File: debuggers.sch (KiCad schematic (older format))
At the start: 7 parts, among them P1 TI_JTAG, P2 SWD, P3 TI_jtag, P4 SWD+SWO+UART

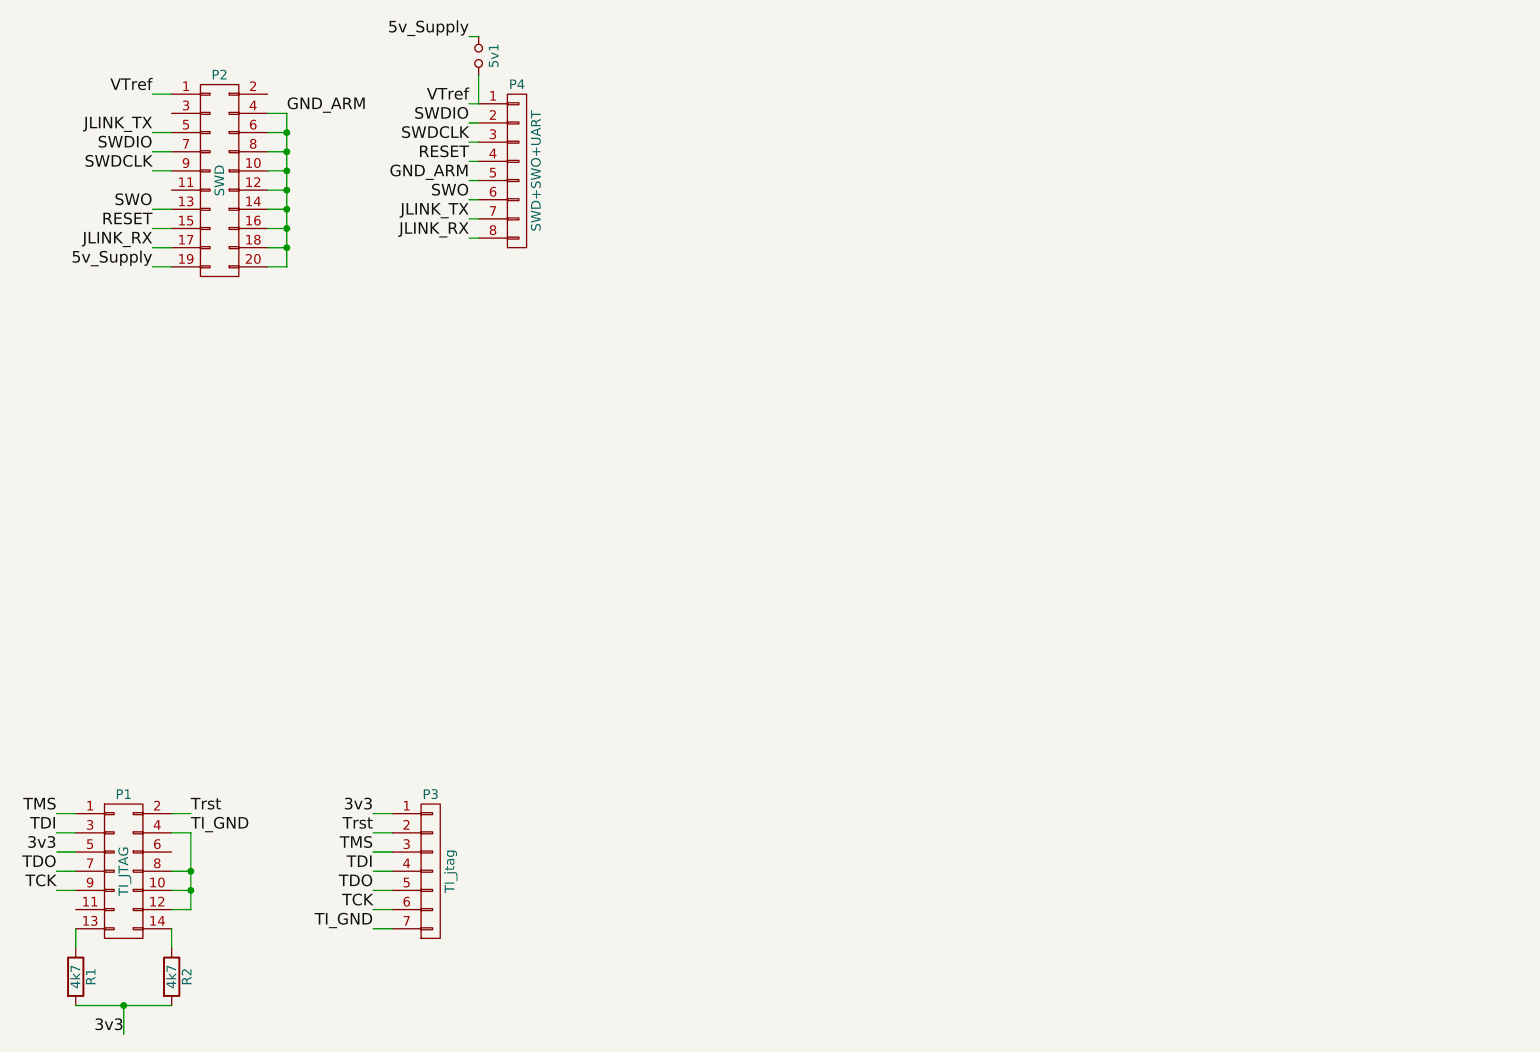
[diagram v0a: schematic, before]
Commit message: Added schematics
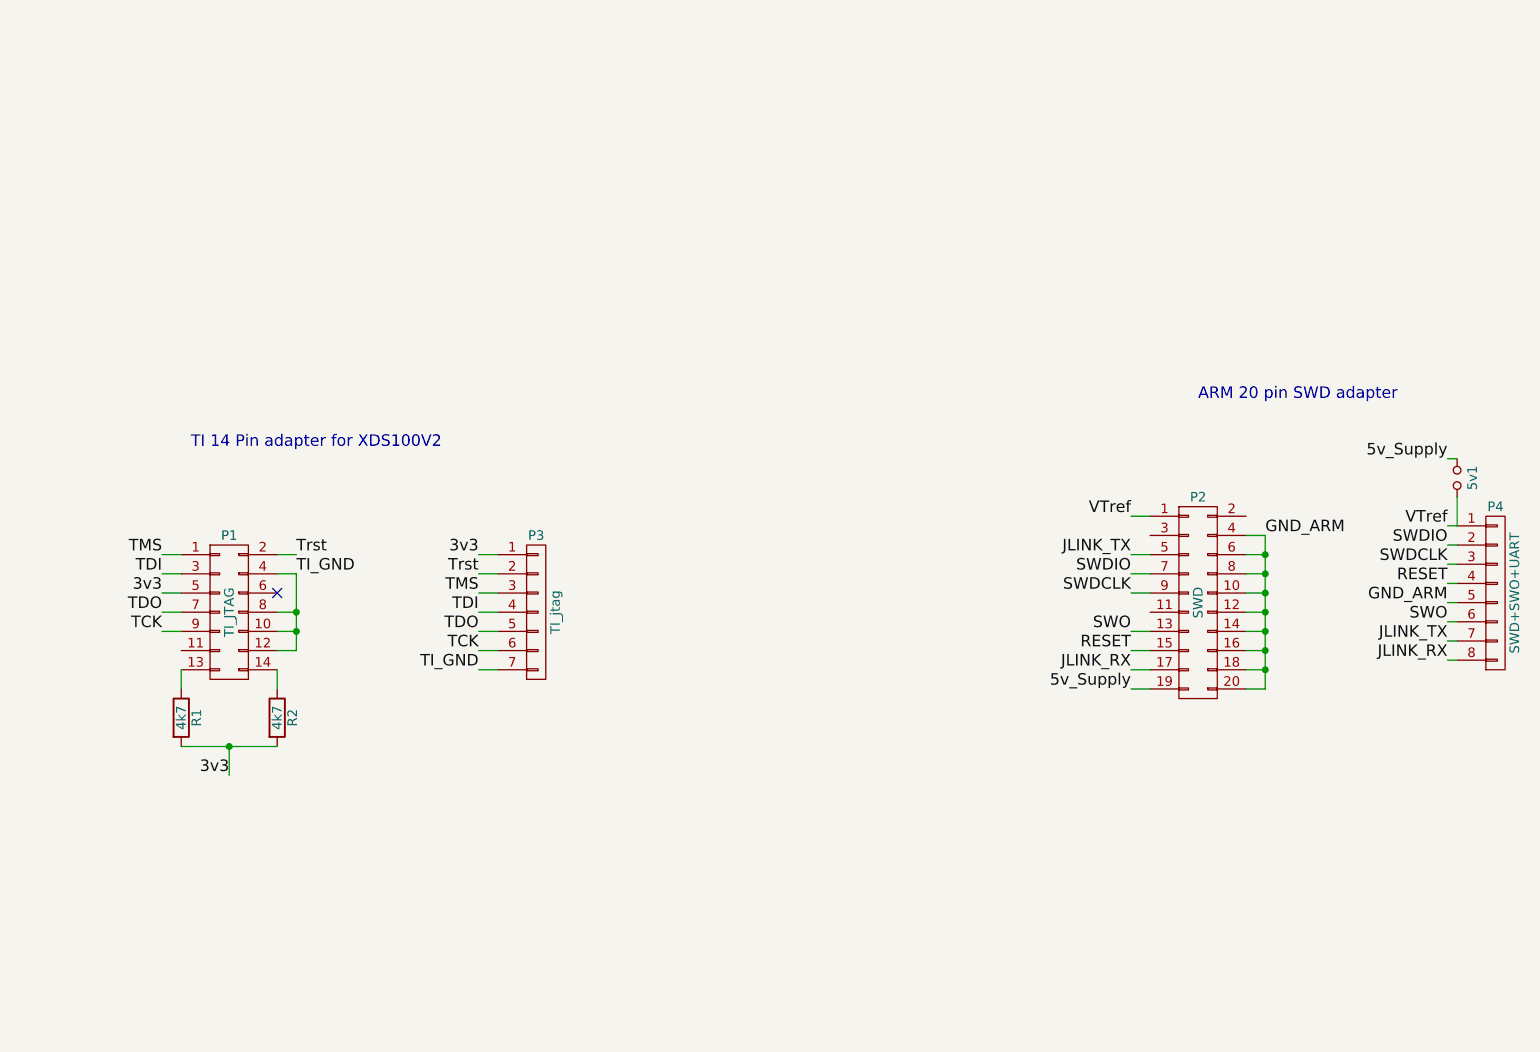
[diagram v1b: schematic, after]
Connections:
- no-connect marks 0 -> 1
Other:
- note added: "ARM 20 pin SWD adapter"
- note added: "TI 14 Pin adapter for XDS100V2"
- moved on the sheet: 5v1, P1, P2, P3, P4, R1, R2

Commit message: Created Seperate boards for each debugger
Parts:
- 5v1: footprint Pin_Headers:Pin_Header_Straight_1x02 -> Pin_Headers:Pin_Header_Straight_1x02_Pitch2.54mm
- P1: footprint Pin_Headers:Pin_Header_Straight_2x07 -> Pin_Headers:Pin_Header_Straight_1x02_Pitch2.00mm
- P2: footprint Pin_Headers:Pin_Header_Straight_2x10 -> Pin_Headers:Pin_Header_Straight_2x10_Pitch2.54mm
- P3: footprint Pin_Headers:Pin_Header_Straight_1x07 -> Pin_Headers:Pin_Header_Straight_1x29_Pitch2.00mm_SMD_Pin1Right
- P4: footprint Pin_Headers:Pin_Header_Straight_1x08 -> Pin_Headers:Pin_Header_Straight_1x08_Pitch2.54mm
- R1, R2: footprint Resistors_SMD:R_1206_HandSoldering -> Relays_THT:Relay_SPDT_PotterBrumfield_T9AP5D52_12V30A
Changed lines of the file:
@@
 F 0 "P2" H 7800 4150 50  0000 C CNN
 F 1 "SWD" V 7800 3600 50  0000 C CNN
-F 2 "Pin_Headers:Pin_Header_Straight_2x10" H 7800 2400 50  0001 C CNN
+F 2 "Pin_Headers:Pin_Header_Straight_2x10_Pitch2.54mm" H 7800 2400 50  0001 C CNN
 F 3 "" H 7800 2400 50  0000 C CNN
 	1    7800 3600
@@
 F 0 "P1" H 2750 4050 50  0000 C CNN
 F 1 "TI_JTAG" V 2750 3650 50  0000 C CNN
-F 2 "Pin_Headers:Pin_Header_Straight_2x07" H 2750 2450 50  0001 C CNN
+F 2 "Pin_Headers:Pin_Header_Straight_1x02_Pitch2.00mm" H 2750 2450 50  0001 C CNN
 F 3 "" H 2750 2450 50  0000 C CNN
 	1    2750 3650
@@
 F 0 "P3" H 4350 4050 50  0000 C CNN
 F 1 "TI_jtag" V 4450 3650 50  0000 C CNN
-F 2 "Pin_Headers:Pin_Header_Straight_1x07" H 4350 3650 50  0001 C CNN
+F 2 "Pin_Headers:Pin_Header_Straight_1x29_Pitch2.00mm_SMD_Pin1Right" H 4350 3650 50  0001 C CNN
 F 3 "" H 4350 3650 50  0000 C CNN
 	1    4350 3650
@@
 F 0 "P4" H 9350 4000 50  0000 C CNN
 F 1 "SWD+SWO+UART" V 9450 3550 50  0000 C CNN
-F 2 "Pin_Headers:Pin_Header_Straight_1x08" H 9350 3550 50  0001 C CNN
+F 2 "Pin_Headers:Pin_Header_Straight_1x08_Pitch2.54mm" H 9350 3550 50  0001 C CNN
 F 3 "" H 9350 3550 50  0000 C CNN
 	1    9350 3550
@@
 F 0 "5v1" H 9150 3030 50  0000 C CNN
 F 1 "Jumper_NO_Small" H 9160 2890 50  0001 C CNN
-F 2 "Pin_Headers:Pin_Header_Straight_1x02" H 9150 2950 50  0001 C CNN
+F 2 "Pin_Headers:Pin_Header_Straight_1x02_Pitch2.54mm" H 9150 2950 50  0001 C CNN
 F 3 "" H 9150 2950 50  0000 C CNN
 	1    9150 2950
@@
 F 0 "R1" V 2580 4200 50  0000 C CNN
 F 1 "4k7" V 2500 4200 50  0000 C CNN
-F 2 "Resistors_SMD:R_1206_HandSoldering" V 2430 4200 50  0001 C CNN
+F 2 "Relays_THT:Relay_SPDT_PotterBrumfield_T9AP5D52_12V30A" V 2430 4200 50  0001 C CNN
 F 3 "" H 2500 4200 50  0000 C CNN
 	1    2500 4200
@@
 F 0 "R2" V 3080 4200 50  0000 C CNN
 F 1 "4k7" V 3000 4200 50  0000 C CNN
-F 2 "Resistors_SMD:R_1206_HandSoldering" V 2930 4200 50  0001 C CNN
+F 2 "Relays_THT:Relay_SPDT_PotterBrumfield_T9AP5D52_12V30A" V 2930 4200 50  0001 C CNN
 F 3 "" H 3000 4200 50  0000 C CNN
 	1    3000 4200

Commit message: Updated layouts
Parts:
- P1: footprint Pin_Headers:Pin_Header_Straight_1x02_Pitch2.00mm -> Pin_Headers:Pin_Header_Straight_2x07_Pitch2.54mm
- P3: footprint Pin_Headers:Pin_Header_Straight_1x29_Pitch2.00mm_SMD_Pin1Right -> Pin_Headers:Pin_Header_Straight_1x07_Pitch2.54mm
- R1, R2: footprint Relays_THT:Relay_SPDT_PotterBrumfield_T9AP5D52_12V30A -> Resistors_SMD:R_1206_HandSoldering
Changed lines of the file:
@@
 F 0 "P1" H 2750 4050 50  0000 C CNN
 F 1 "TI_JTAG" V 2750 3650 50  0000 C CNN
-F 2 "Pin_Headers:Pin_Header_Straight_1x02_Pitch2.00mm" H 2750 2450 50  0001 C CNN
+F 2 "Pin_Headers:Pin_Header_Straight_2x07_Pitch2.54mm" H 2750 2450 50  0001 C CNN
 F 3 "" H 2750 2450 50  0000 C CNN
 	1    2750 3650
@@
 F 0 "P3" H 4350 4050 50  0000 C CNN
 F 1 "TI_jtag" V 4450 3650 50  0000 C CNN
-F 2 "Pin_Headers:Pin_Header_Straight_1x29_Pitch2.00mm_SMD_Pin1Right" H 4350 3650 50  0001 C CNN
+F 2 "Pin_Headers:Pin_Header_Straight_1x07_Pitch2.54mm" H 4350 3650 50  0001 C CNN
 F 3 "" H 4350 3650 50  0000 C CNN
 	1    4350 3650
@@
 F 0 "R1" V 2580 4200 50  0000 C CNN
 F 1 "4k7" V 2500 4200 50  0000 C CNN
-F 2 "Relays_THT:Relay_SPDT_PotterBrumfield_T9AP5D52_12V30A" V 2430 4200 50  0001 C CNN
+F 2 "Resistors_SMD:R_1206_HandSoldering" V 2430 4200 50  0001 C CNN
 F 3 "" H 2500 4200 50  0000 C CNN
 	1    2500 4200
@@
 F 0 "R2" V 3080 4200 50  0000 C CNN
 F 1 "4k7" V 3000 4200 50  0000 C CNN
-F 2 "Relays_THT:Relay_SPDT_PotterBrumfield_T9AP5D52_12V30A" V 2930 4200 50  0001 C CNN
+F 2 "Resistors_SMD:R_1206_HandSoldering" V 2930 4200 50  0001 C CNN
 F 3 "" H 3000 4200 50  0000 C CNN
 	1    3000 4200
